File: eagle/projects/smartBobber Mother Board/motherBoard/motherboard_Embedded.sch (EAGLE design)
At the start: 29 parts, among them Q1 2A/20V/150mΩ, Q2 MMBT3904, Y1 ECS-40-S-4X

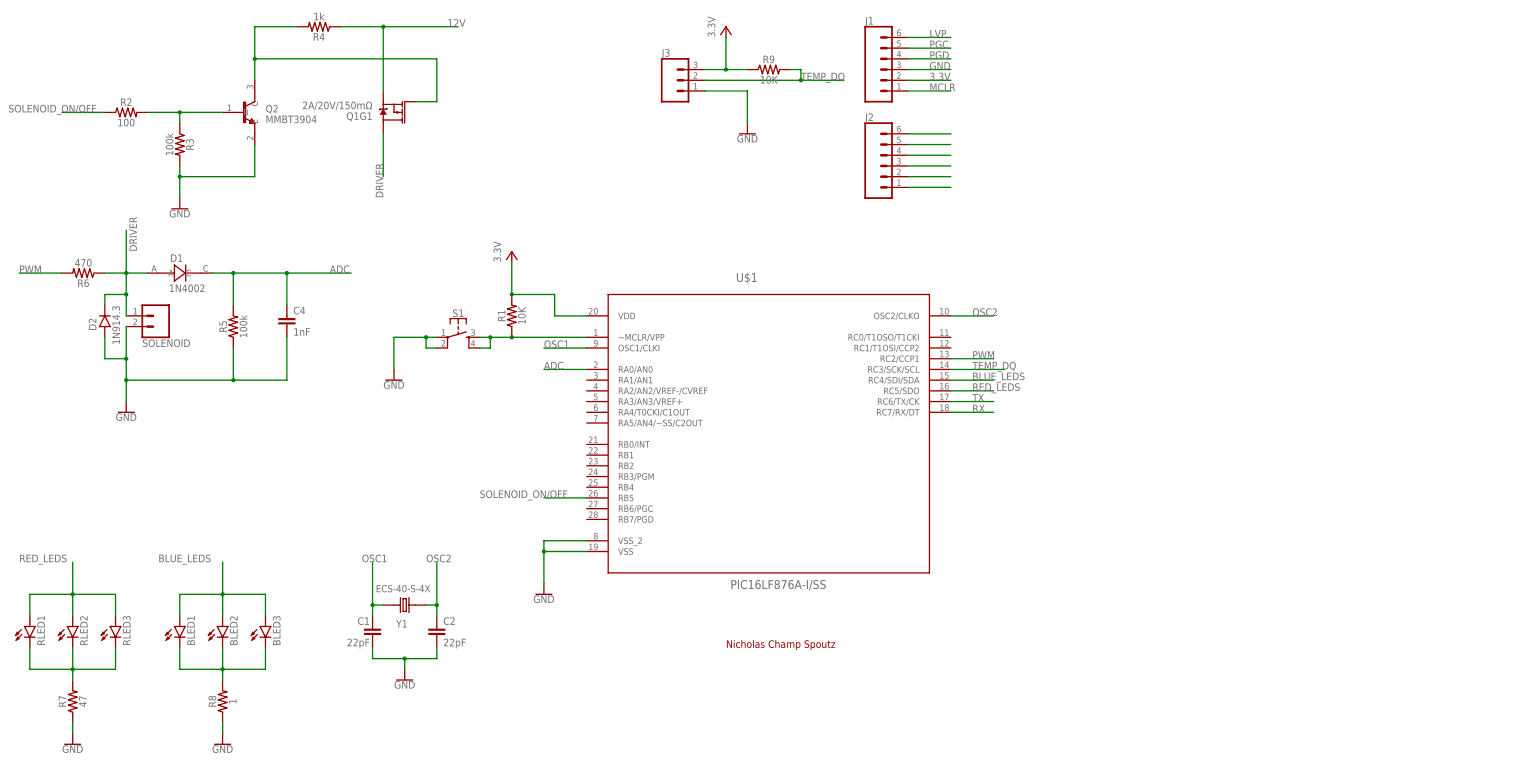
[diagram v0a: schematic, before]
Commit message: Update motherboard_Embedded.sch
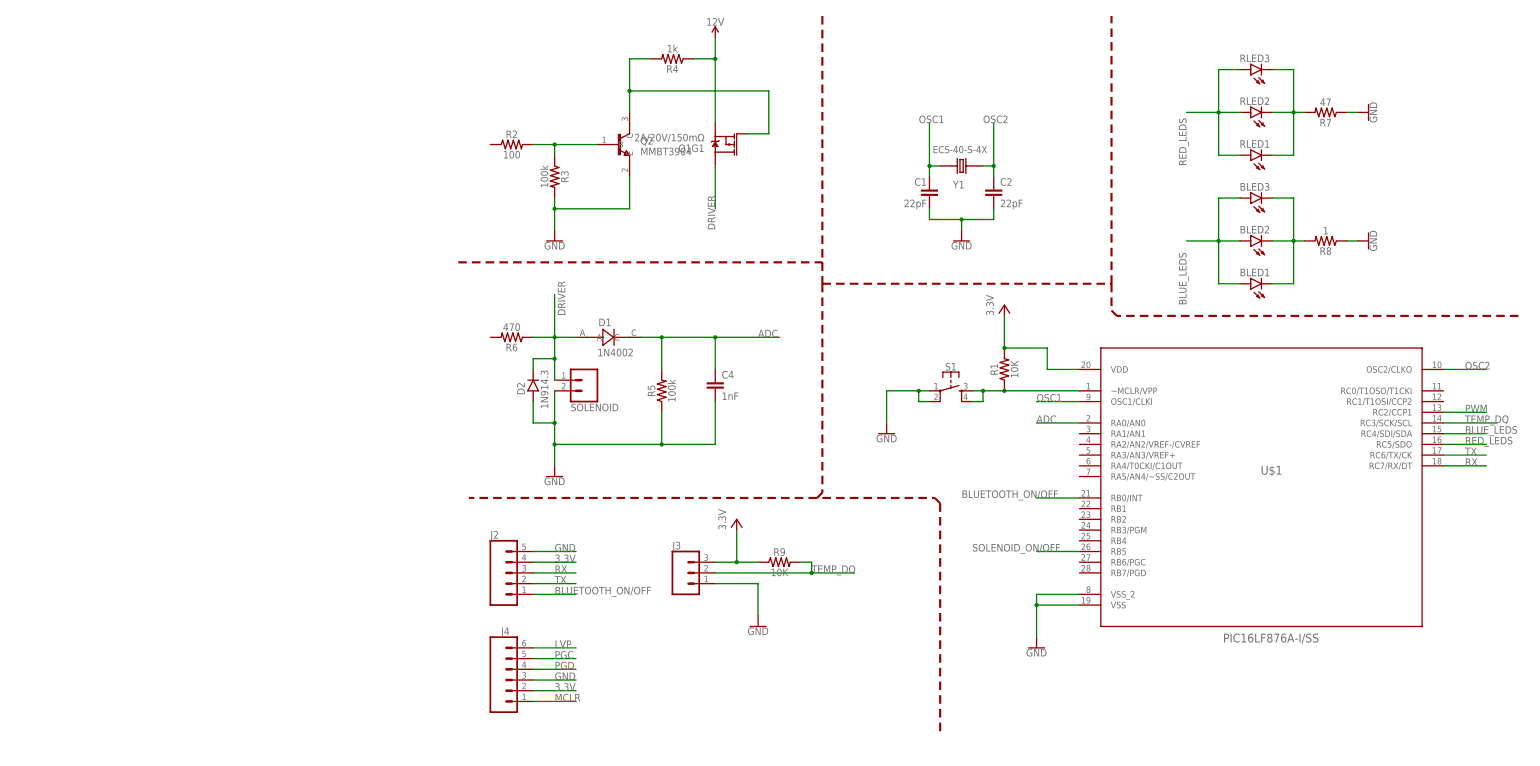
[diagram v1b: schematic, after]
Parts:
- removed J1: (no value), SparkFun-Connectors:CONN_06POLAR
- added J4: (no value), SparkFun-Connectors:CONN_06SILK_FEMALE_PTH
- J2: device SparkFun-Connectors:CONN_06POLAR -> SparkFun-Connectors:CONN_05JST-VERT
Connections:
- removed net 12V: Q1G1.S, R4.1
- removed net N$11: J2.6
- removed net N$12: J2.5
- removed net N$13: J2.4
- removed net N$14: J2.3
- removed net N$15: J2.2
- removed net N$16: J2.1
- new net BLUETOOTH_ON/OFF: J2.1, U$1.RB0/INT
- net 3.3V: now also J2.4, J4.2; no longer J1.2
- net GND: now also J2.5, J4.3; no longer J1.3
- net LVP: now also J4.6; no longer J1.6
- net MCLR: now also J4.1; no longer J1.1
- net PGC: now also J4.5; no longer J1.5
- net PGD: now also J4.4; no longer J1.4
- net PWM: no longer R6.2
- net RX: now also J2.3
- net SOLENOID_ON/OFF: no longer R2.1
- net TX: now also J2.2
- net VCC: now also Q1G1.S, R4.1
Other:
- note removed: "Nicholas Champ Spoutz"
- moved on the sheet: BLED1, BLED2, BLED3, C1, C2, C4, D1, D2, J3, Q1G1, Q2, R1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

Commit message: Update motherboard_Embedded.sch
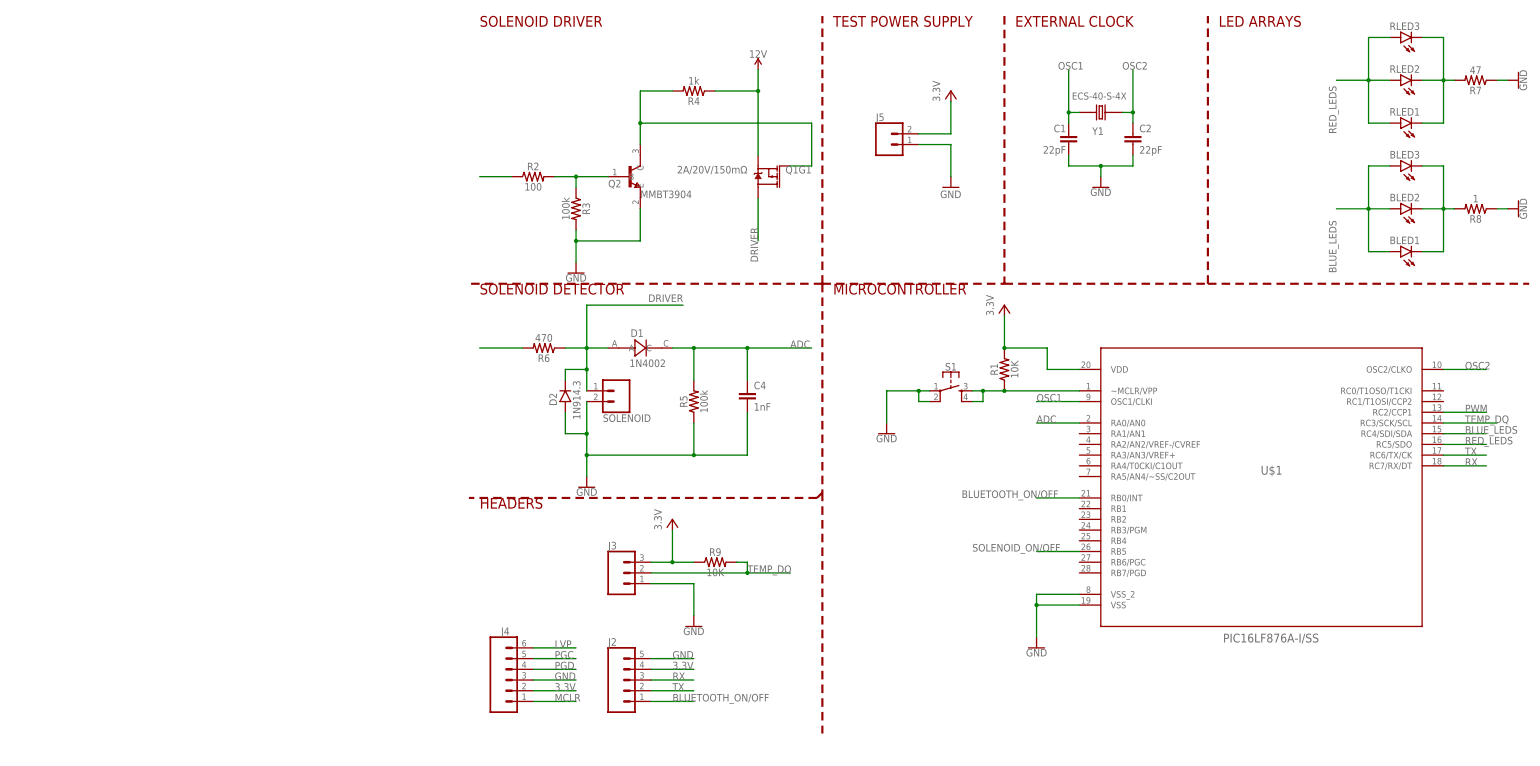
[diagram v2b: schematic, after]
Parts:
- added J5: (no value), SparkFun-Connectors:CONN_02
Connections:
- new net N$2: R6.2
- new net N$7: R2.1
- net GND: now also J5.1
- net VCC: now also J5.2
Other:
- note added: "EXTERNAL CLOCK"
- note added: "HEADERS"
- note added: "LED ARRAYS"
- note added: "MICROCONTROLLER"
- note added: "SOLENOID DETECTOR"
- note added: "SOLENOID DRIVER"
- note added: "TEST POWER SUPPLY"
- moved on the sheet: BLED1, BLED2, BLED3, C1, C2, C4, D1, D2, J2, J3, Q1G1, Q2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
